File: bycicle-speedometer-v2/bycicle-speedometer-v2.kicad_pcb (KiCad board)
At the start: 2 copper layers, 58 x 30 mm, 23 parts, among them J1 Conn_01x02_Pin, J2 Conn_01x02_Pin, J3 Conn_01x02_Pin, J4 Conn_01x03_Pin, SW1 SW_Push_Dual, U1 ESP-12E

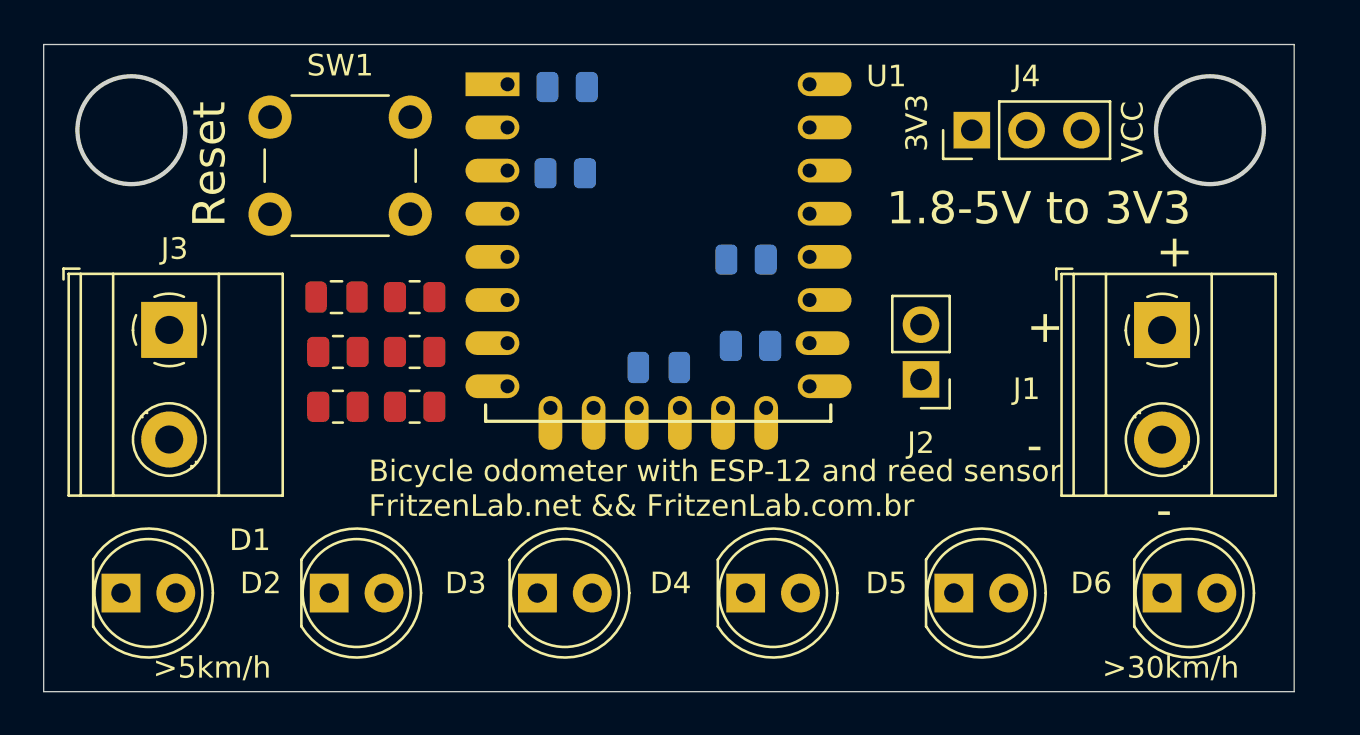
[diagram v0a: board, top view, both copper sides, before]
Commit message: created fabrication files
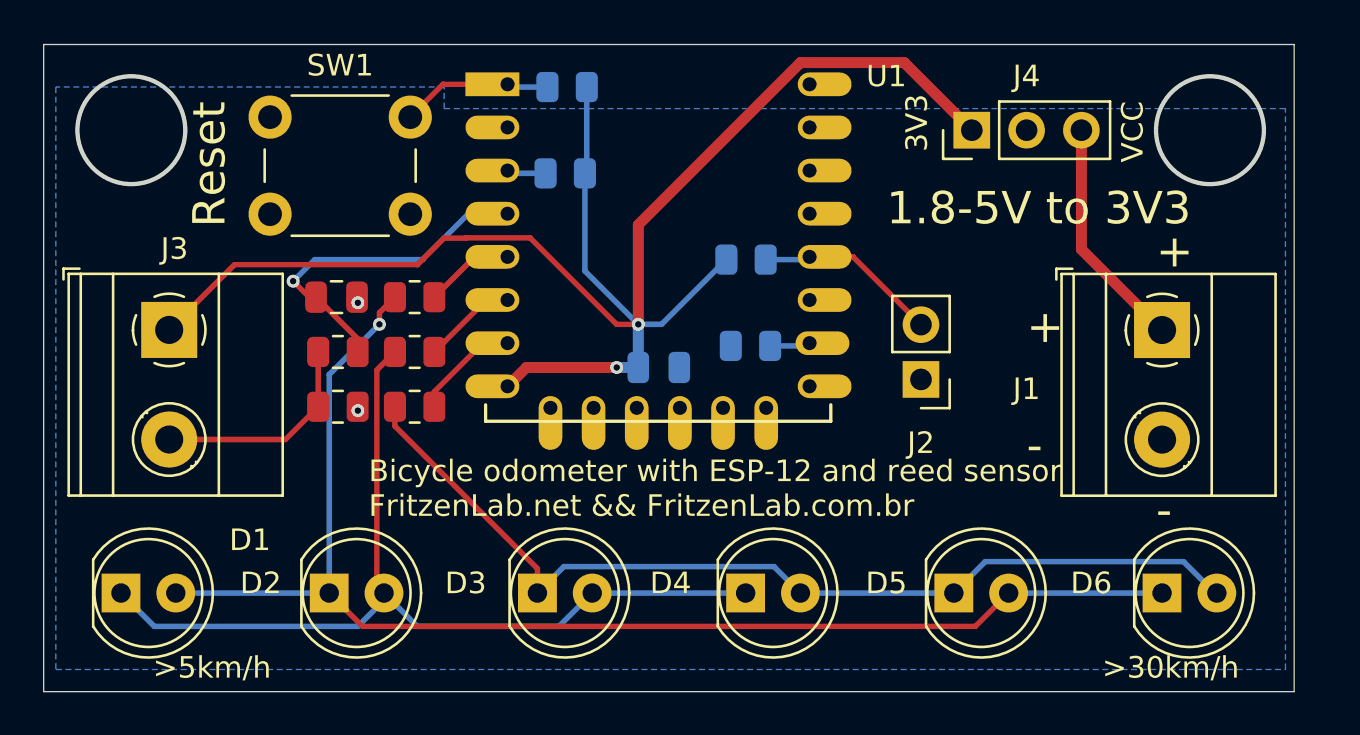
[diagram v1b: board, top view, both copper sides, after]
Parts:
- R5: value R -> 10k
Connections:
- C1 pad 1: Net-(U1-VCC) -> 3V3
- U1 pad 8: Net-(U1-VCC) -> 3V3
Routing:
- net 3V3: track 0.00 -> 75.8 mm, vias 0 -> 2
- net Net-(D1-A): track 0.00 -> 62.0 mm, vias 0 -> 1
- net Net-(D3-K): track 0.00 -> 45.1 mm
- net Net-(D1-K): track 0.00 -> 43.4 mm
- net Sensor: track 0.00 -> 15.9 mm, vias 0 -> 1
- net VCC: track 0.00 -> 10.8 mm
- net Net-(J3-Pin_2): track 0.00 -> 10.1 mm
- net Prog: track 0.00 -> 8.55 mm
- net Net-(U1-REST): track 0.00 -> 7.04 mm
- net led_c: track 0.00 -> 5.02 mm
- net led_b: track 0.00 -> 4.39 mm
- net led_a: track 0.00 -> 4.17 mm
- net Net-(U1-GPIO15): track 0.00 -> 1.88 mm
- net Net-(U1-CH_PD): track 0.00 -> 1.81 mm
- net GND: vias 0 -> 2
- added copper zone on B.Cu, net GND
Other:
- board text added: "FritzenLab.net && FritzenLab.com.br"
- board text added: "Reed switch here ->"
- board text removed: "Reed sensor here ->"
